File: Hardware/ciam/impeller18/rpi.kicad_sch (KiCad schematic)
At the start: 12 parts, among them J7 Raspberry Pi 4

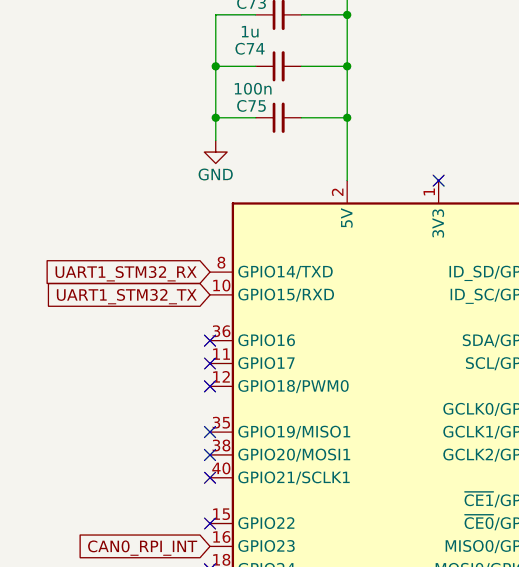
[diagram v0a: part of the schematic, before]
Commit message: updatec schematics
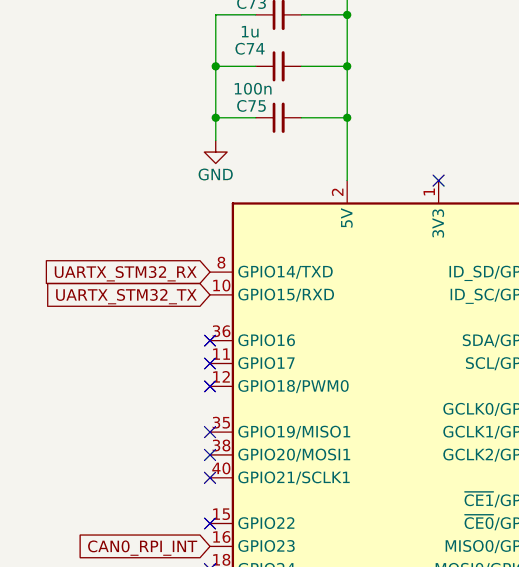
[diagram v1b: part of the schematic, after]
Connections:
- net UART1_STM32_RX renamed UARTX_STM32_RX
- net UART1_STM32_TX renamed UARTX_STM32_TX
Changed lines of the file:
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@@
 		)
 	)
-	(global_label "UART1_STM32_TX"
+	(global_label "UARTX_STM32_TX"
 		(shape input)
 		(at 170.18 95.885 180)
@@
 				)
 				(justify left)
-				(hide yes)
-			)
-		)
-	)
-	(global_label "UART1_STM32_RX"
-		(shape input)
-		(at 170.18 93.345 180)
-		(fields_autoplaced yes)
-		(effects
-			(font
-				(size 1.27 1.27)
-			)
-			(justify right)
-		)
-		(property "Intersheetrefs" "${INTERSHEET_REFS}"
-			(at 150.8664 93.345 0)
-			(effects
-				(font
-					(size 1.27 1.27)
-				)
-				(justify right)
 				(hide yes)
 			)
@@
 				(hide yes)
 			)
+		)
+	)
+	(global_label "UARTX_STM32_RX"
+		(shape input)
+		(at 170.18 93.345 180)
+		(fields_autoplaced yes)
+		(effects
+			(font
+				(size 1.27 1.27)
+			)
+			(justify right)
+		)
+		(property "Intersheetrefs" "${INTERSHEET_REFS}"
+			(at 150.8664 93.345 0)
+			(effects
+				(font
+					(size 1.27 1.27)
+				)
+				(justify right)
+				(hide yes)
+			)

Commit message: added footprints
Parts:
- C73, C74, C75: footprint (none) -> Capacitor_SMD:C_0603_1608Metric
- D12, D13: footprint (none) -> user_lib:LED_RGB_promelec
- R35, R36, R37, R38, R39, R40: footprint (none) -> Resistor_SMD:R_0603_1608Metric
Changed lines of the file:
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@@
 			)
 		)
-		(property "Footprint" ""
+		(property "Footprint" "user_lib:LED_RGB_promelec"
 			(at 273.685 127.635 0)
 			(effects
@@
 			)
 		)
-		(property "Footprint" ""
+		(property "Footprint" "Resistor_SMD:R_0603_1608Metric"
 			(at 285.115 128.143 90)
 			(effects
@@
 			)
 		)
-		(property "Footprint" ""
+		(property "Footprint" "Capacitor_SMD:C_0603_1608Metric"
 			(at 177.8 70.485 0)
 			(effects
@@
 			)
 		)
-		(property "Footprint" ""
+		(property "Footprint" "Capacitor_SMD:C_0603_1608Metric"
 			(at 177.8 64.77 0)
 			(effects
@@
 			)
 		)
-		(property "Footprint" ""
+		(property "Footprint" "user_lib:LED_RGB_promelec"
 			(at 273.685 100.33 0)
 			(effects
@@
 			)
 		)
-		(property "Footprint" ""
+		(property "Footprint" "Resistor_SMD:R_0603_1608Metric"
 			(at 285.115 133.223 90)
 			(effects
@@
 			)
 		)
-		(property "Footprint" ""
+		(property "Footprint" "Resistor_SMD:R_0603_1608Metric"
 			(at 285.115 100.838 90)
 			(effects
@@
 			)
 		)
-		(property "Footprint" ""
+		(property "Footprint" "Resistor_SMD:R_0603_1608Metric"
 			(at 285.115 105.918 90)
 			(effects
@@
 			)
 		)
-		(property "Footprint" ""
+		(property "Footprint" "Capacitor_SMD:C_0603_1608Metric"
 			(at 177.8 76.2 0)
 			(effects
@@
 			)
 		)
-		(property "Footprint" ""
+		(property "Footprint" "Resistor_SMD:R_0603_1608Metric"
 			(at 285.115 95.758 90)
 			(effects
@@
 			)
 		)
-		(property "Footprint" ""
+		(property "Footprint" "Resistor_SMD:R_0603_1608Metric"
 			(at 285.115 123.063 90)
 			(effects

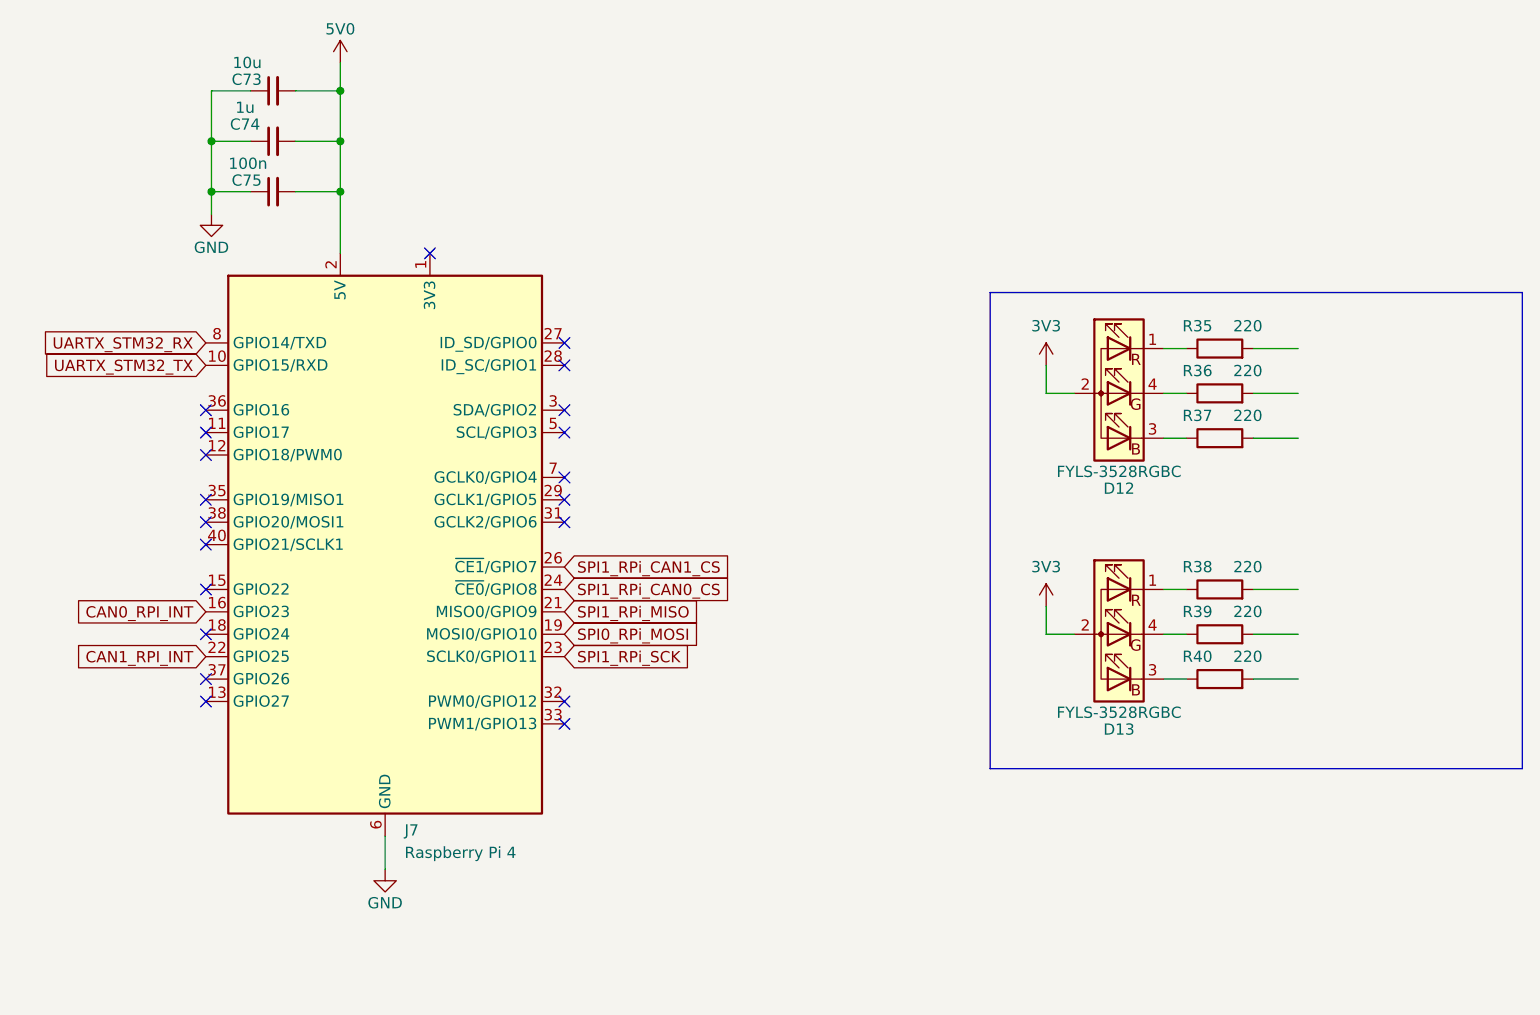
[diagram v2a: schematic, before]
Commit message: Minor changes
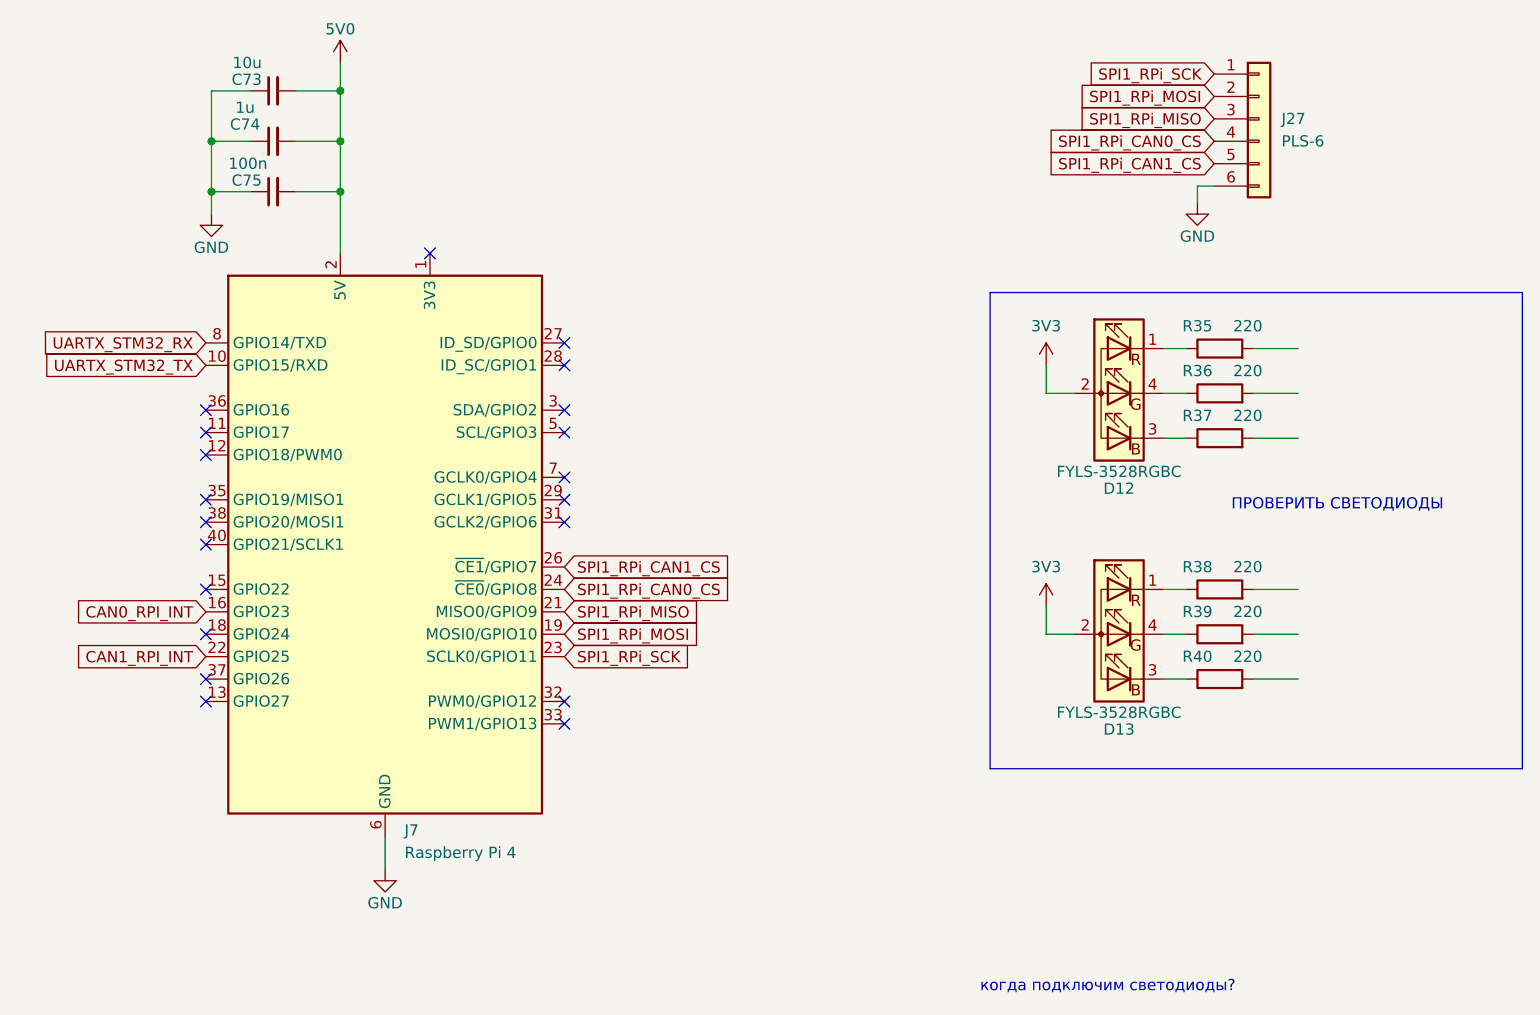
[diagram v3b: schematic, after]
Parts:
- added J27: PLS-6, Connector_PinHeader_2.54mm:PinHeader_1x06_P2.54mm_Vertical, symbol Connector_Generic:Conn_01x06
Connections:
- net GND: now also J27.6 (Pin_6)
- net SPI1_RPi_CAN0_CS: now also J27.4 (Pin_4)
- net SPI1_RPi_CAN1_CS: now also J27.5 (Pin_5)
- net SPI1_RPi_MISO: now also J27.3 (Pin_3)
- net SPI1_RPi_SCK: now also J27.1 (Pin_1)
- net SPI0_RPi_MOSI renamed SPI1_RPi_MOSI
- net SPI1_RPi_MOSI: now also J27.2 (Pin_2)
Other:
- note added: "ПРОВЕРИТЬ СВЕТОДИОДЫ"
- note added: "когда подключим светодиоды?"
